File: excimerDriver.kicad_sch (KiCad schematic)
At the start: 37 parts, among them IC3 INA210, IC6 STM32G071KBT6, J1 B08B-XASK-1-A_LF__SN_, J2 TC2050-IDC, J3 BM02B-SRSS-TB_LF__SN_, J4 BM02B-SRSS-TB_LF__SN_, J6 640445-2, Q3 BSS138

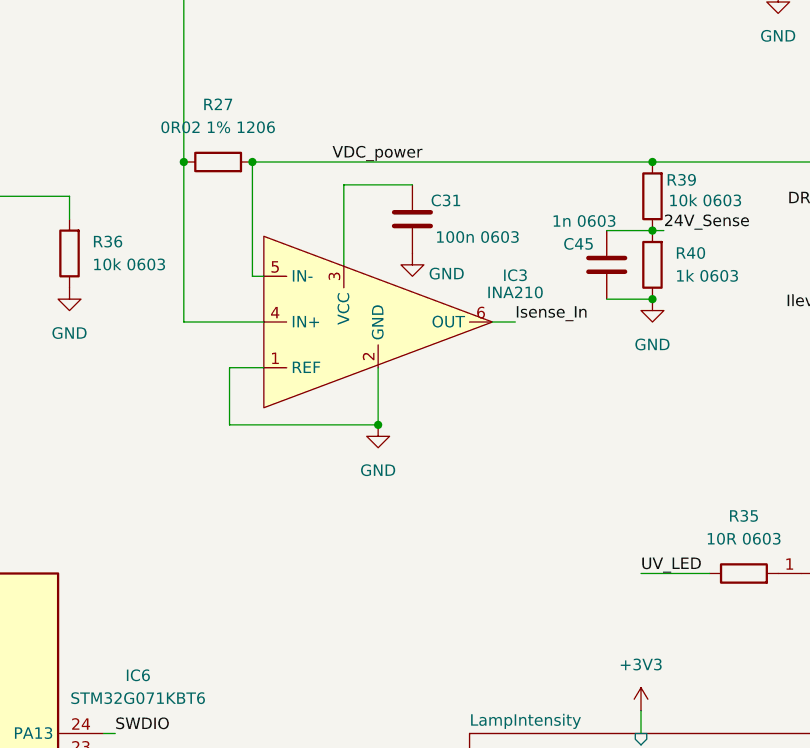
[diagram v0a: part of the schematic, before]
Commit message: 251704 end of day
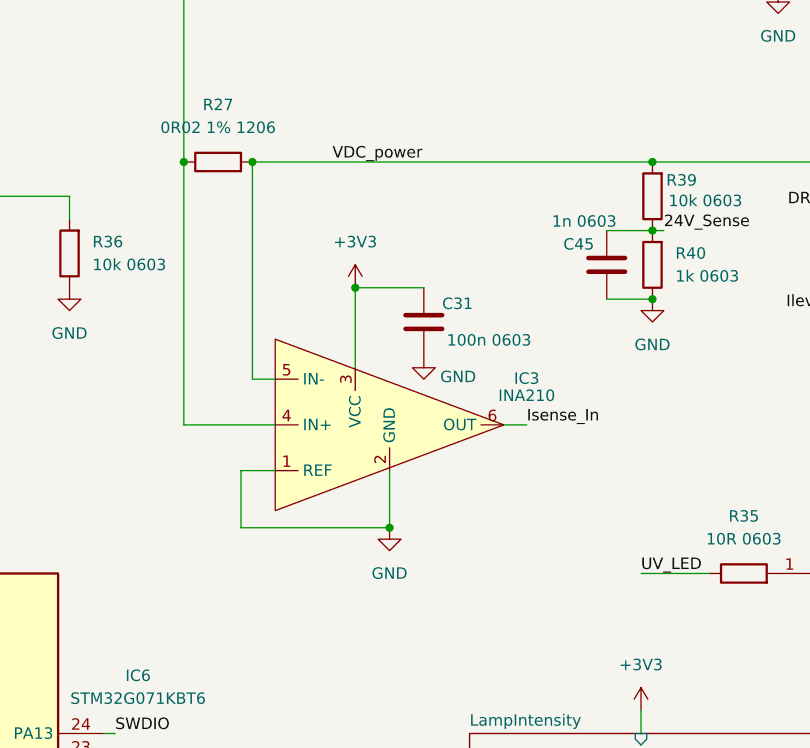
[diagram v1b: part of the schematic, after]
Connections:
- net +3V3: now also C31.1, IC3.3 (VCC)
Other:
- moved on the sheet: C31, IC3
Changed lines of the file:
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@@
 	)
 	(junction
+		(at 148.59 77.47)
+		(diameter 0)
+		(color 0 0 0 0)
+	)
+	(junction
 		(at 43.18 148.59)
 		(diameter 0)
@@
 	)
 	(junction
-		(at 151.13 92.71)
+		(at 152.4 104.14)
 		(diameter 0)
 		(color 0 0 0 0)
@@
 	(wire
 		(pts
-			(xy 151.13 86.36) (xy 151.13 92.71)
+			(xy 152.4 97.79) (xy 152.4 104.14)
 		)
 		(stroke
@@
 	(wire
 		(pts
-			(xy 137.16 76.2) (xy 138.43 76.2)
+			(xy 137.16 87.63) (xy 139.7 87.63)
 		)
 		(stroke
@@
 	(wire
 		(pts
-			(xy 137.16 63.5) (xy 137.16 76.2)
+			(xy 137.16 63.5) (xy 137.16 87.63)
 		)
 		(stroke
@@
 	(wire
 		(pts
-			(xy 147.32 66.04) (xy 154.94 66.04)
+			(xy 148.59 77.47) (xy 156.21 77.47)
 		)
 		(stroke
@@
 	(wire
 		(pts
-			(xy 134.62 86.36) (xy 134.62 92.71)
+			(xy 135.89 97.79) (xy 135.89 104.14)
 		)
 		(stroke
@@
 	(wire
 		(pts
-			(xy 147.32 74.93) (xy 147.32 66.04)
+			(xy 148.59 86.36) (xy 148.59 77.47)
 		)
 		(stroke
@@
 	(wire
 		(pts
-			(xy 134.62 92.71) (xy 151.13 92.71)
+			(xy 135.89 104.14) (xy 152.4 104.14)
 		)
 		(stroke
@@
 	(wire
 		(pts
-			(xy 138.43 86.36) (xy 134.62 86.36)
+			(xy 139.7 97.79) (xy 135.89 97.79)
 		)
 		(stroke
@@
 	(wire
 		(pts
-			(xy 129.54 81.28) (xy 138.43 81.28)
+			(xy 129.54 92.71) (xy 139.7 92.71)
 		)
 		(stroke
@@
 	(wire
 		(pts
-			(xy 129.54 63.5) (xy 129.54 81.28)
+			(xy 129.54 63.5) (xy 129.54 92.71)
 		)
 		(stroke
@@
 	(wire
 		(pts
-			(xy 163.83 81.28) (xy 166.37 81.28)
+			(xy 165.1 92.71) (xy 167.64 92.71)
 		)
 		(stroke
@@
 			"UFgAAAAAMSgsAAAAgBgUFgAAAEAMCgsAAAAgBoUFAAAAEIPCAgAAAIhBYQEAAADEoLAAAAAAYlBY"
 			"AAAAADEoLAAAAIAYFBYAAABADAoLAAAAIAaFBQAAABCDwgIAAACIQWEBAAAAxKCwAAAAAGL+FzCI"
-			"XY5DdsKkAAAAAElFTkSuQmCC"
+			"XY5DdsKkAAAAAElFTkSuQmCC+P////////9IxoOeIgEAAPj/////////KM6DniIBAAD4////////"
+			"/7jOg54iAQAA+P////////8EAAAAIgEAAPj/////////AAAAACIBAAD4/////////3id7MoiAQAA"
+			"+P////////8EAAAAIgEAAPj/////////QOn1lSIBAAD4/////////wQAAAAiAQAA+P////////9o"
+			"0IOeIgEAAPj/////////cOv1lSIBAAD4//////////DS9ZUiAQAA+P////////8EAAAAIgEAAPj/"
+			"////////BAAAACIBAAD4/////////wQAAAAiAQAA+P////////8AAAAAIgEAAPj/////////QNv1"
+			"lSIBAAD4//////////Dn9ZUiAQAA+P////////8A3fWVIgEAAPj/////////BAAAACIBAAD4////"
+			"/////8De9ZUiAQAA+P////////8EAAAAIgEAAPj/////////BAAAACIBAAD4/////////wQAAAAi"
+			"AQAA+P////////+CBAAAIgEAAPj/////////BAAAACIBAAD4/////////+h97MoiAQAA+P//////"
+			"//8EAAAAIgEAAPj/////////BAAAACIBAAD4/////////zDR9ZUiAQAA+P////////8EAAAAIgEA"
+			"APj/////////BAAAACIBAAD4/////////8De9ZUiAQAA+P////////8EAAAAIgEAAPj/////////"
+			"IOr1lSIBAAD4/////////yDq9ZUiAQAA+P////////8EAAAAIgEAAPj/////////BAAAACIBAAD4"
+			"/////////8DQ9ZUiAQAA+P////////8EAAAAIgEAAPj/////////BAAAACIBAAD4/////////wQA"
+			"AAAiAQAA+P////////8AAAAAIgEAAPj/////////OLiDniIBAAD4/////////wQAAAAiAQAA+P//"
+			"//////9Q5fWVIgEAAPj/////////MAQAACIBAAD4/////////1i5g54iAQAA+P////////8EAAAA"
+			"IgEAAPj/////////aIDsyiIBAAD4/////////wQAAAAiAQAA+P////////8EAAAAIgEAAPj/////"
+			"////CJ/syiIBAAD4/////////wQAAAAiAQAA+P////////8oczLTIgEAAPj/////////BAAAACIB"
+			"AAD4/////////yhzMtMiAQAA+P////////8EAAAAIgEAAPj/////////BAAAACIBAAD4////////"
+			"/yhzMtMiAQAA+P////////8EAAAAIgEAAPj/////////KHMy0yIBAAD4/////////yhzMtMiAQAA"
+			"+P////////8EAAAAIgEAAA=="
 		)
 	)
@@
 	)
 	(label "Isense_In"
-		(at 166.37 81.28 0)
+		(at 167.64 92.71 0)
 		(effects
 			(font
@@
 	(symbol
 		(lib_id "power:GND")
-		(at 154.94 73.66 0)
+		(at 156.21 85.09 0)
 		(unit 1)
 		(exclude_from_sim no)
@@
 		(dnp no)
 		(property "Reference" "#PWR030"
-			(at 154.94 80.01 0)
+			(at 156.21 91.44 0)
 			(hide yes)
 			(effects
@@
 		)
 		(property "Value" "GND"
-			(at 158.75 75.946 0)
+			(at 160.02 87.376 0)
 			(effects
 				(font
@@
 		)
 		(property "Footprint" ""
-			(at 154.94 73.66 0)
+			(at 156.21 85.09 0)
 			(hide yes)
 			(effects
@@
 		)
 		(property "Datasheet" ""
-			(at 154.94 73.66 0)
+			(at 156.21 85.09 0)
 			(hide yes)
 			(effects
@@
 		)
 		(property "Description" "Power symbol creates a global label with name \"GND\" , ground"
-			(at 154.94 73.66 0)
+			(at 156.21 85.09 0)
 			(hide yes)
 			(effects
@@
 	)
 	(symbol
+		(lib_id "power:+3V3")
+		(at 148.59 77.47 0)
+		(unit 1)
+		(exclude_from_sim no)
+		(in_bom yes)
+		(on_board yes)
+		(dnp no)
+		(fields_autoplaced yes)
+		(property "Reference" "#PWR082"
+			(at 148.59 81.28 0)
+			(hide yes)
+			(effects
+				(font
+					(size 1.27 1.27)
+				)
+			)
+		)
+		(property "Value" "+3V3"
+			(at 148.59 72.39 0)
+			(effects
+				(font
+					(size 1.27 1.27)
+				)
+			)
+		)
+		(property "Footprint" ""
+			(at 148.59 77.47 0)
+			(hide yes)
+			(effects
+				(font
+					(size 1.27 1.27)
+				)
+			)
+		)
+		(property "Datasheet" ""
+			(at 148.59 77.47 0)
+			(hide yes)
+			(effects
+				(font
+					(size 1.27 1.27)
+				)
+			)
+		)
+		(property "Description" "Power symbol creates a global label with name \"+3V3\""
+			(at 148.59 77.47 0)
+			(hide yes)
+			(effects
+				(font
+					(size 1.27 1.27)
+				)
+			)
+		)
+		(pin "1"
+		)
+		(instances
+			(project "OSLUV"
+				(path "/c6e900e0-9399-44f0-8089-9dd7b8ffe54c/9b3070c3-43e0-4d43-9da1-9bc1bd2d6fb9"
+					(reference "#PWR082")
+					(unit 1)
+				)
+			)
+		)
+	)
+	(symbol
 		(lib_id "power:GND")
 		(at 55.88 121.92 0)
@@
 	(symbol
 		(lib_id "Device:C")
-		(at 154.94 69.85 0)
+		(at 156.21 81.28 0)
 		(unit 1)
 		(exclude_from_sim no)
@@
 		(dnp no)
 		(property "Reference" "C31"
-			(at 156.972 67.818 0)
+			(at 158.242 79.248 0)
 			(effects
 				(font
@@
 		)
 		(property "Value" "100n 0603"
-			(at 157.48 71.882 0)
+			(at 158.75 83.312 0)
 			(effects
 				(font
@@
 		)
 		(property "Footprint" "Capacitor_SMD:C_0603_1608Metric"
-			(at 155.9052 73.66 0)
+			(at 157.1752 85.09 0)
 			(hide yes)
 			(effects
@@
 		)
 		(property "Datasheet" ""
-			(at 154.94 69.85 0)
+			(at 156.21 81.28 0)
 			(hide yes)
 			(effects
@@
 		)
 		(property "Description" "Unpolarized capacitor"
-			(at 154.94 69.85 0)
+			(at 156.21 81.28 0)
 			(hide yes)
 			(effects
@@
 	(symbol
 		(lib_id "power:GND")
-		(at 151.13 92.71 0)
+		(at 152.4 104.14 0)
 		(unit 1)
 		(exclude_from_sim no)
@@
 		(fields_autoplaced yes)
 		(property "Reference" "#PWR029"
-			(at 151.13 99.06 0)
+			(at 152.4 110.49 0)
 			(hide yes)
 			(effects
@@
 		)
 		(property "Value" "GND"
-			(at 151.13 97.79 0)
+			(at 152.4 109.22 0)
 			(effects
 				(font
@@
 		)
 		(property "Footprint" ""
-			(at 151.13 92.71 0)
+			(at 152.4 104.14 0)
 			(hide yes)
 			(effects
@@
 		)
 		(property "Datasheet" ""
-			(at 151.13 92.71 0)
+			(at 152.4 104.14 0)
 			(hide yes)
 			(effects
@@
 		)
 		(property "Description" "Power symbol creates a global label with name \"GND\" , ground"
-			(at 151.13 92.71 0)
+			(at 152.4 104.14 0)
 			(hide yes)
 			(effects
@@
 	(symbol
 		(lib_id "Hansmann:INA210")
-		(at 138.43 81.28 0)
+		(at 139.7 92.71 0)
 		(unit 1)
 		(exclude_from_sim no)
@@
 		(fields_autoplaced yes)
 		(property "Reference" "IC3"
-			(at 166.37 76.1298 0)
+			(at 167.64 87.5598 0)
 			(effects
 				(font
@@
 		)
 		(property "Value" "INA210"
-			(at 166.37 78.0349 0)
+			(at 167.64 89.4649 0)
 			(effects
 				(font
@@
 		)
 		(property "Footprint" "Hansmann:SOT95P280X90-6N"
-			(at 138.43 81.28 0)
+			(at 139.7 92.71 0)
 			(hide yes)
 			(effects
@@
 		)
 		(property "Datasheet" ""
-			(at 138.43 81.28 0)
+			(at 139.7 92.71 0)
 			(hide yes)
 			(effects
@@
 		)
 		(property "Description" ""
-			(at 138.43 81.28 0)
+			(at 139.7 92.71 0)
 			(hide yes)
 			(effects
